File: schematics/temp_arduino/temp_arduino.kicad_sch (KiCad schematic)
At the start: 3 parts

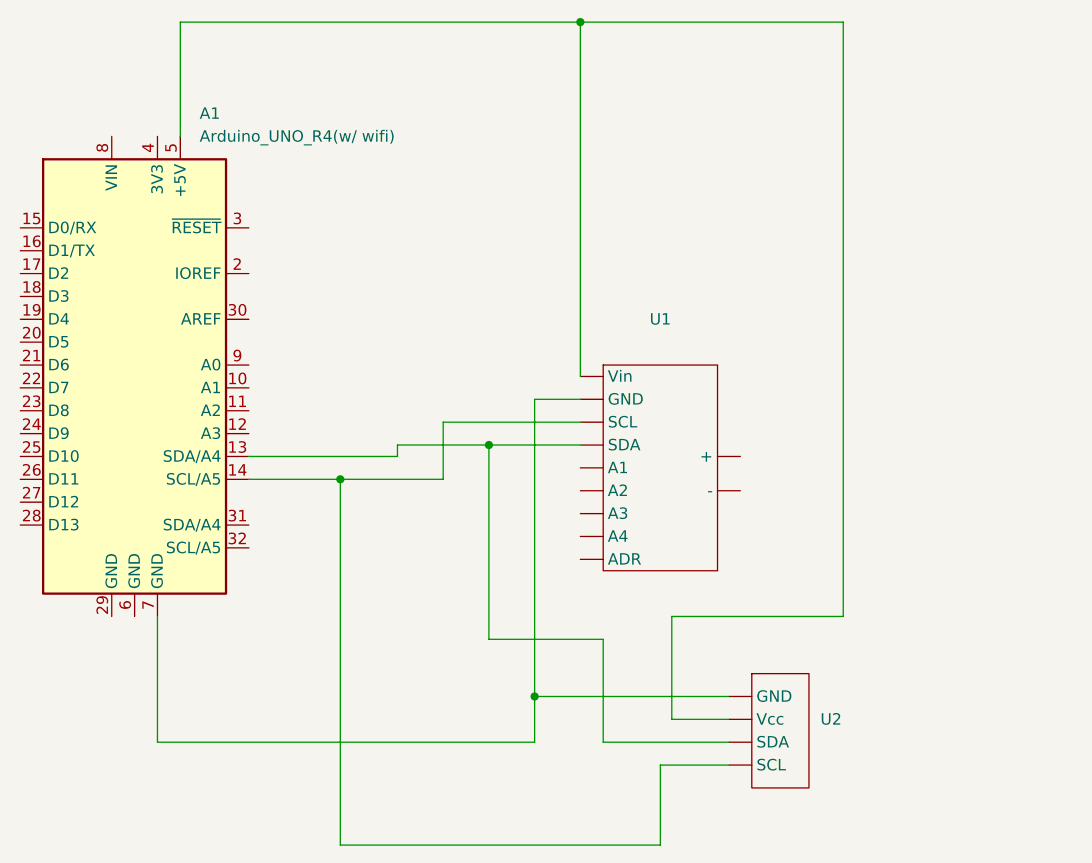
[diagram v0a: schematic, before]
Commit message: update schematics
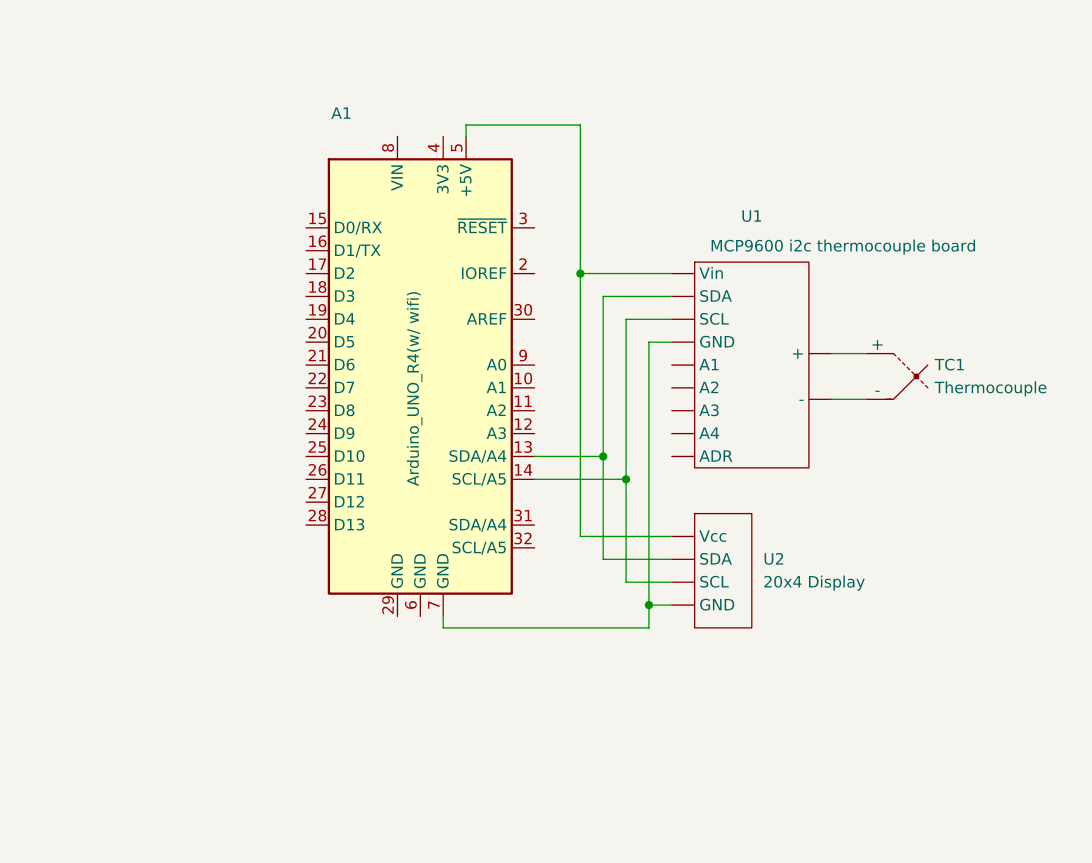
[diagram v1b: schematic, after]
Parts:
- added TC1: Thermocouple, symbol Device:Thermocouple
- U1: value ~ -> MCP9600 i2c thermocouple board
- U2: value ~ -> 20x4 Display
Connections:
- net at U1. (-): now also TC1.2 (-)
- new net: A1.13 (SDA/A4), U1. (-), U2. (GND)
- new net: A1.14 (SCL/A5), U1. (-), U2. (GND)
- new net: A1.5 (+5V), U1. (-), U2. (GND)
- new net: TC1.1 (+), U1. (-)
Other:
- moved on the sheet: A1, U1, U2
